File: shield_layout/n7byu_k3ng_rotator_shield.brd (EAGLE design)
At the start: 67 x 63.5 mm, 27 parts, among them J1 ARDUINO_R3_SHIELD, J10 ROTCABLE, J2 EL, J3 AZ, J4 ELToggle, J5 I2C-OLD, J6 I2C-NEW, J7 RST, J8 PARK, J9 STOP, Q1 2N3904, Q2 2N3904, Q3 2N3904, Q4 2N3904

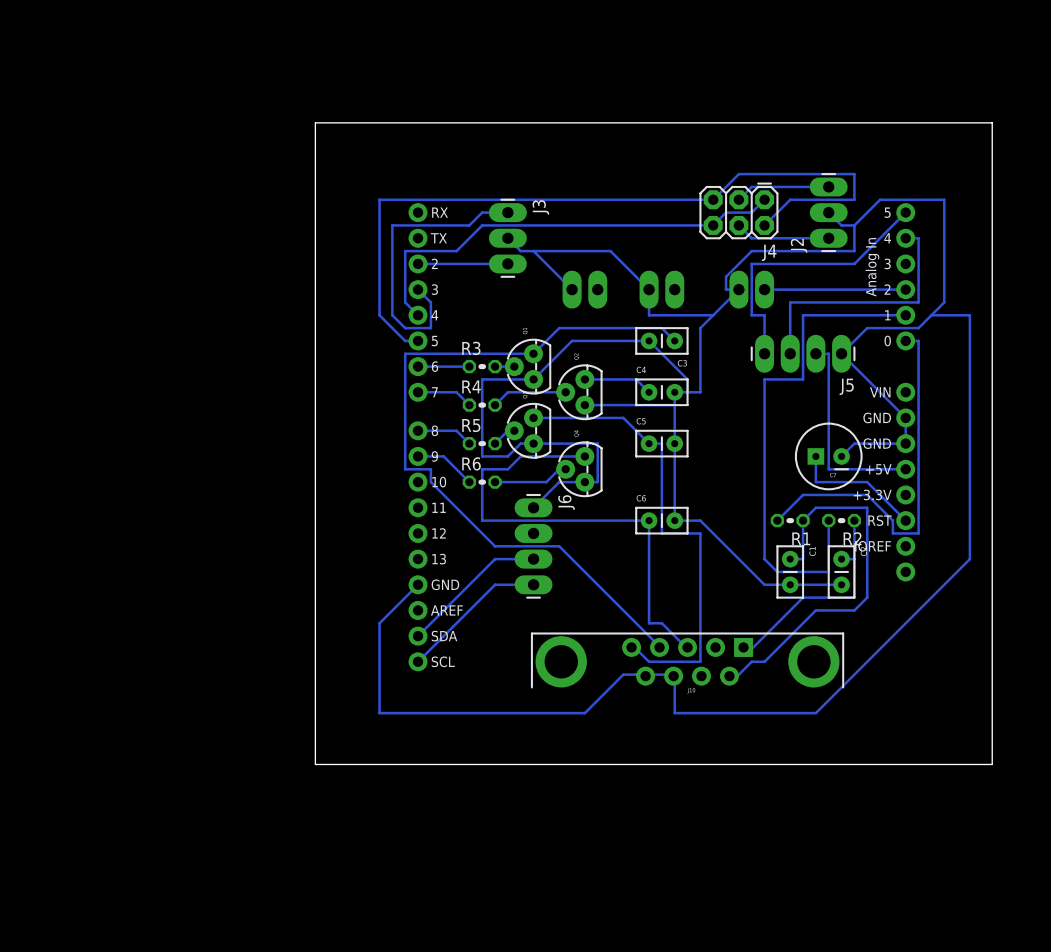
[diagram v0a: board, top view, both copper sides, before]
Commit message: got it down to 3 jumpers on one layer. still working...
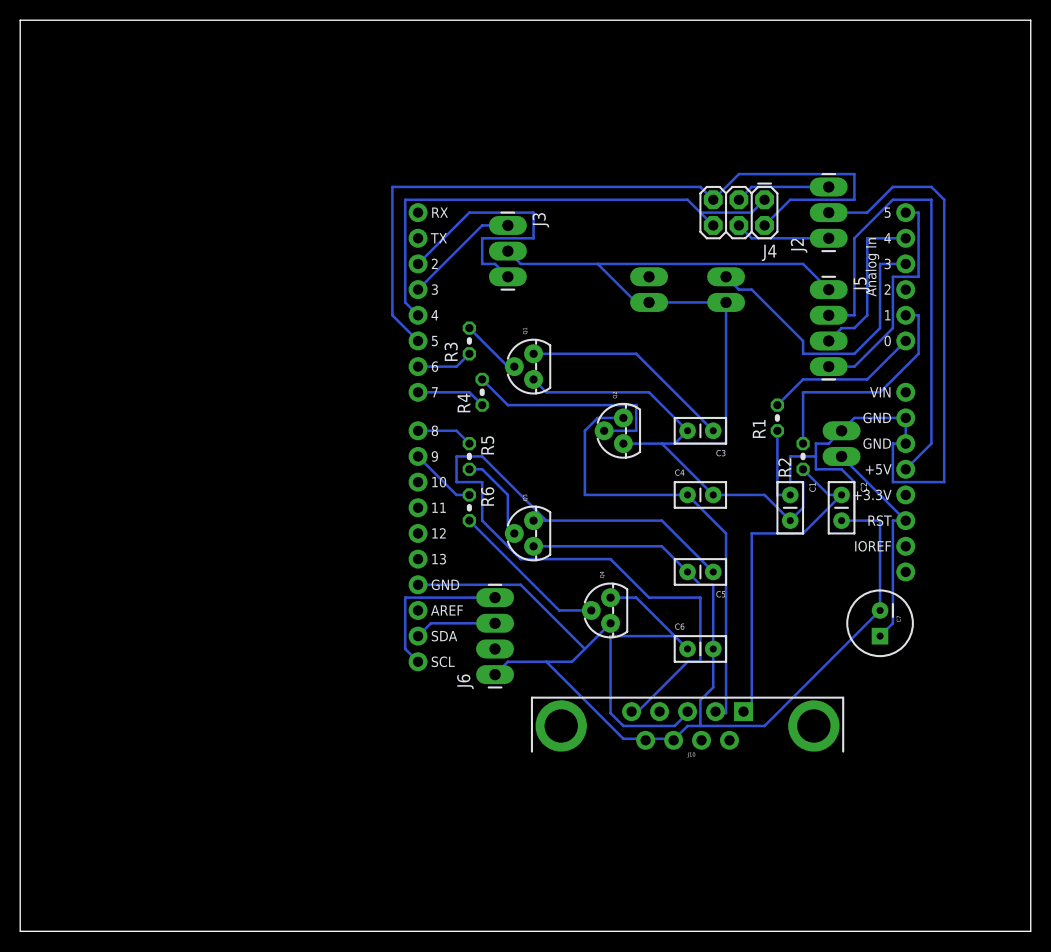
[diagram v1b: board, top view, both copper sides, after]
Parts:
- moved J7 29.2 mm to (81.3, 47.0), turned to 90 degrees
- moved C7 17.3 mm to (85.1, 30.5), turned to 270 degrees
- moved J6 16.9 mm to (47.0, 25.4), turned to 90 degrees
- moved C5 14.2 mm to (68.6, 35.6), turned to 180 degrees
- moved Q4 14.2 mm to (58.4, 31.8)
- moved C6 13.3 mm to (66.0, 27.9)
- moved J9 11.5 mm to (62.2, 64.8), turned to 270 degrees
- moved C4 10.9 mm to (66.0, 43.2)
- moved R1 10.2 mm to (74.9, 50.8), turned to 90 degrees
- moved Q3 10.2 mm to (50.8, 39.4)
- moved C3 9.67 mm to (68.6, 49.5)
- moved R2 7.41 mm to (77.5, 47.0), turned to 90 degrees
- moved J5 6.48 mm to (80.0, 63.5), turned to 270 degrees
- moved C1 6.35 mm to (76.2, 43.2)
- moved C2 6.35 mm to (81.3, 43.2)
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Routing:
- net N$9: track 73.5 -> 20.9 mm
- net N$10: track 6.88 -> 45.6 mm
- net N$18: track 46.5 -> 80.3 mm
- net N$1: track 37.6 -> 7.62 mm
- net N$28: track 0.00 -> 29.1 mm
- net N$6: track 50.1 -> 23.2 mm
- net N$26: track 20.3 -> 47.1 mm
- net N$4: track 37.7 -> 15.3 mm
- net CCW-BUTTON: track 29.5 -> 11.5 mm
- net CW-BUTTON: track 8.89 -> 26.8 mm
- net N$12: track 47.4 -> 32.5 mm
- net N$3: track 7.51 -> 22.0 mm
- net N$22: track 14.0 -> 0.00 mm
- net GND: track 326.1 -> 312.6 mm
- net N$5: track 22.0 -> 33.9 mm
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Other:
- board size 67 x 63.5 mm -> 100 x 90.2 mm
